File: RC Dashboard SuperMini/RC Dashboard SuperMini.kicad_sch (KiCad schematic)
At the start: 8 parts, among them IC1 0.91_I2C_OLED, J5 CH1, J6 CH2

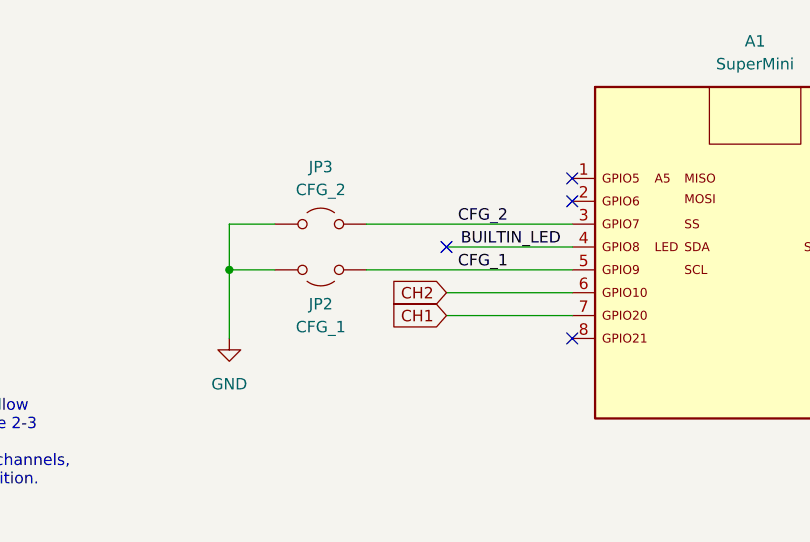
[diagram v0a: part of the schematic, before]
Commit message: Small build tweaks
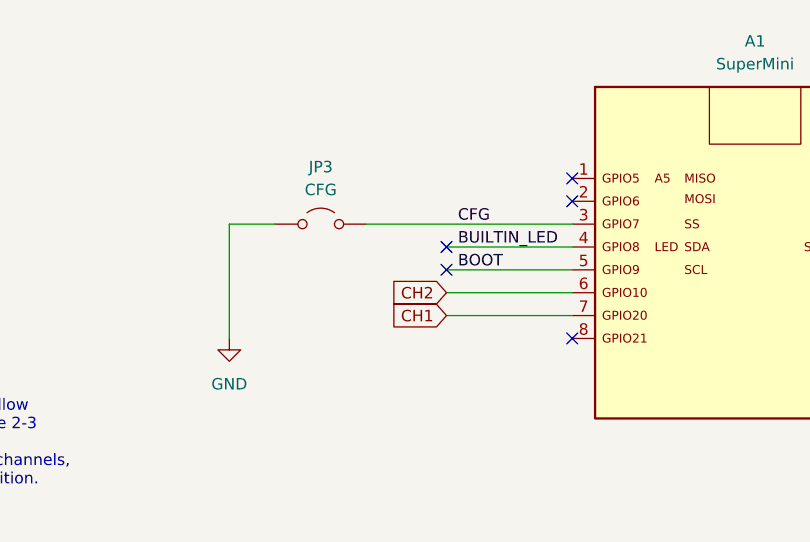
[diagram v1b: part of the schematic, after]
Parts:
- removed JP2: CFG_1, solder_bridge:bridge, symbol Jumper:Jumper_2_Open
- JP3: value CFG_2 -> CFG
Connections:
- net CFG_1 renamed BOOT
- net CFG_2 renamed CFG
- no-connect marks 7 -> 8
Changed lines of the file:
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@@
-	)
-	(junction
-		(at 121.92 88.9)
-		(diameter 0)
-		(color 0 0 0 0)
 	)
 	(junction
@@
 	)
 	(no_connect
+		(at 146.05 88.9)
+	)
+	(no_connect
 		(at 160.02 81.28)
 	)
@@
 	(wire
 		(pts
-			(xy 121.92 88.9) (xy 127 88.9)
-		)
-		(stroke
-			(width 0)
-			(type default)
-		)
-	)
-	(wire
-		(pts
 			(xy 121.92 83.82) (xy 127 83.82)
 		)
@@
 	(wire
 		(pts
-			(xy 121.92 83.82) (xy 121.92 88.9)
+			(xy 121.92 83.82) (xy 121.92 96.52)
 		)
 		(stroke
@@
 	(wire
 		(pts
-			(xy 137.16 88.9) (xy 160.02 88.9)
-		)
-		(stroke
-			(width 0)
-			(type default)
-		)
-	)
-	(wire
-		(pts
 			(xy 71.12 71.12) (xy 71.12 73.66)
 		)
@@
 	(wire
 		(pts
-			(xy 121.92 88.9) (xy 121.92 96.52)
-		)
-		(stroke
-			(width 0)
-			(type default)
-		)
-	)
-	(wire
-		(pts
 			(xy 204.47 68.58) (xy 204.47 78.74)
 		)
@@
 		(pts
 			(xy 208.28 125.73) (xy 208.28 128.27)
+		)
+		(stroke
+			(width 0)
+			(type default)
+		)
+	)
+	(wire
+		(pts
+			(xy 146.05 88.9) (xy 160.02 88.9)
 		)
 		(stroke
@@
 		)
 	)
-	(label "CFG_2"
+	(label "BOOT"
+		(at 147.32 88.9 0)
+		(fields_autoplaced yes)
+		(effects
+			(font
+				(size 1.27 1.27)
+			)
+			(justify left bottom)
+		)
+	)
+	(label "CFG"
 		(at 147.32 83.82 0)
 		(fields_autoplaced yes)
@@
 		)
 	)
-	(label "CFG_1"
-		(at 147.32 88.9 0)
-		(fields_autoplaced yes)
-		(effects
-			(font
-				(size 1.27 1.27)
-			)
-			(justify left bottom)
-		)
-	)
 	(label "SCL"
 		(at 223.52 120.65 180)
@@
 	)
 	(label "BUILTIN_LED"
-		(at 158.75 86.36 180)
+		(at 147.32 86.36 0)
 		(fields_autoplaced yes)
 		(effects
@@
 				(size 1.27 1.27)
 			)
-			(justify right bottom)
+			(justify left bottom)
 		)
 	)
@@
 			)
 		)
-		(property "Value" "CFG_2"
+		(property "Value" "CFG"
 			(at 132.08 80.01 0)
 			(effects
@@
 					(unit 1)
 				)
-			)
-		)
-	)
-	(symbol
-		(lib_id "Jumper:Jumper_2_Open")
-		(at 132.08 88.9 0)
-		(mirror x)
-		(unit 1)
-		(exclude_from_sim yes)
-		(in_bom yes)
-		(on_board yes)
-		(dnp no)
-		(property "Reference" "JP2"
-			(at 132.08 92.71 0)
-			(effects
-				(font
-					(size 1.27 1.27)
-				)
-			)
-		)
-		(property "Value" "CFG_1"
-			(at 132.08 95.25 0)
-			(effects
-				(font
-					(size 1.27 1.27)
-				)
-			)
-		)
-		(property "Footprint" "solder_bridge:bridge"
-			(at 132.08 88.9 0)
-			(effects
-				(font
-					(size 1.27 1.27)
-				)
-				(hide yes)
-			)
-		)
-		(property "Datasheet" "~"
-			(at 132.08 88.9 0)
-			(effects
-				(font
-					(size 1.27 1.27)
-				)
-				(hide yes)
-			)
-		)
-		(property "Description" "Jumper, 2-pole, open"
-			(at 132.08 88.9 0)
-			(effects
-				(font
-					(size 1.27 1.27)
-				)
-				(hide yes)
-			)
-		)
-		(pin "1"
-		)
-		(pin "2"
-		)
-		(instances
-			(project ""
-				(path "/8ea515ea-bab1-45cc-8dd8-41301b605afe"
-					(reference "JP2")
-					(unit 1)
-				)
